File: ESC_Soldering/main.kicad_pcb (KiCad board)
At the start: 2 copper layers, 172 x 77 mm, 29 parts, among them P1 CONN_02X03, P2 CONN_01X03, P3 CONN_01X03, P4 CONN_01X02, P5 CONN_02X05, Q1 BC847CE6327HTSA1, Q2 BC847CE6327HTSA1, U1 PCA9698, U2 ADS7828, U3 AUIPS7111S, U4 AUIPS7111S, U5 74LVC1G08, U6 74LVC1G08, U7 Littlebee, U8 Littlebee

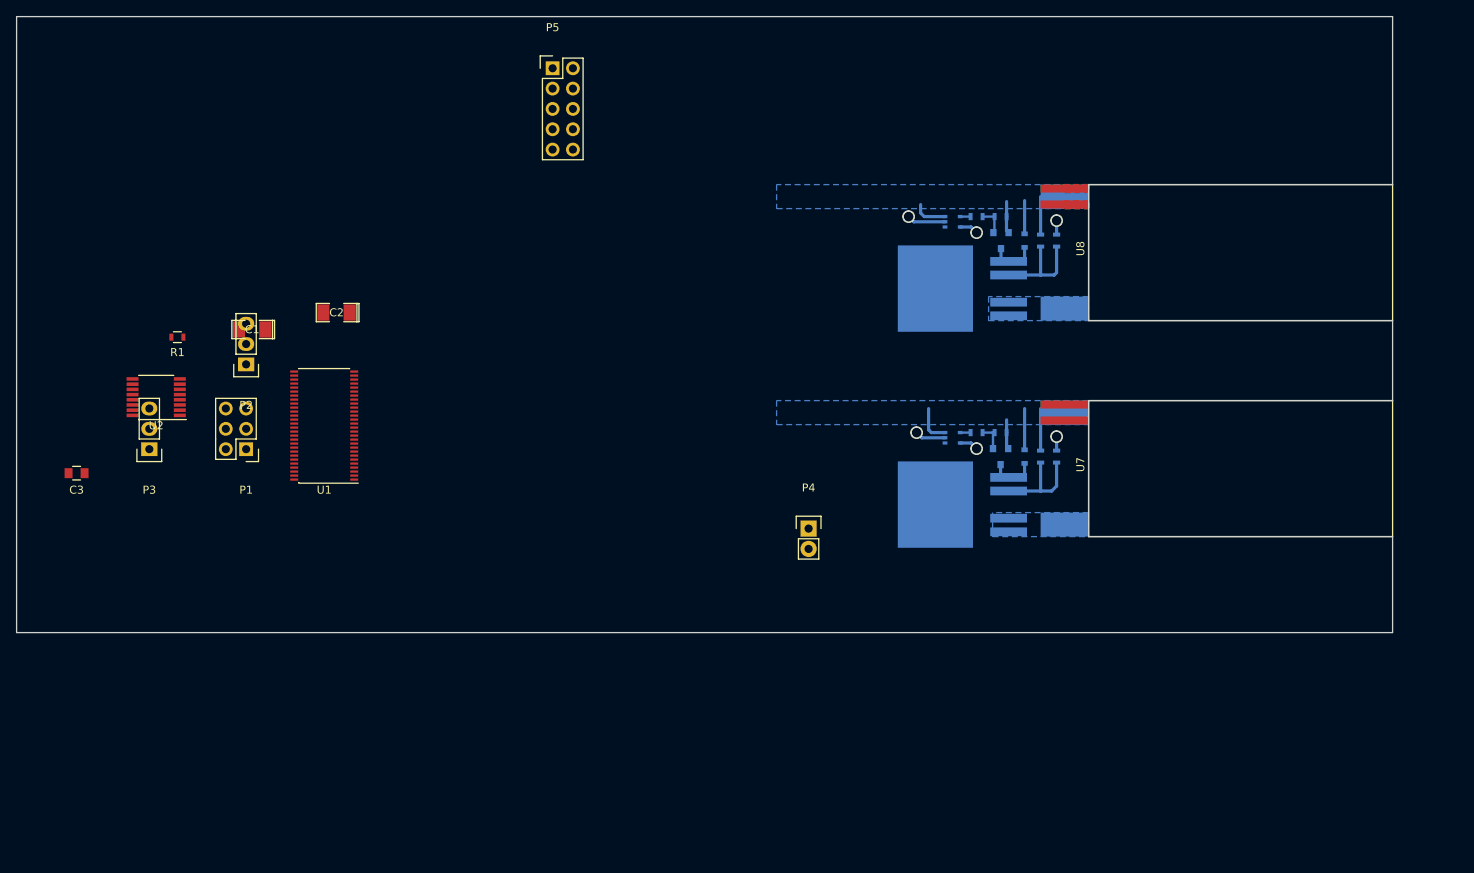
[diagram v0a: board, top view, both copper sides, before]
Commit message: test
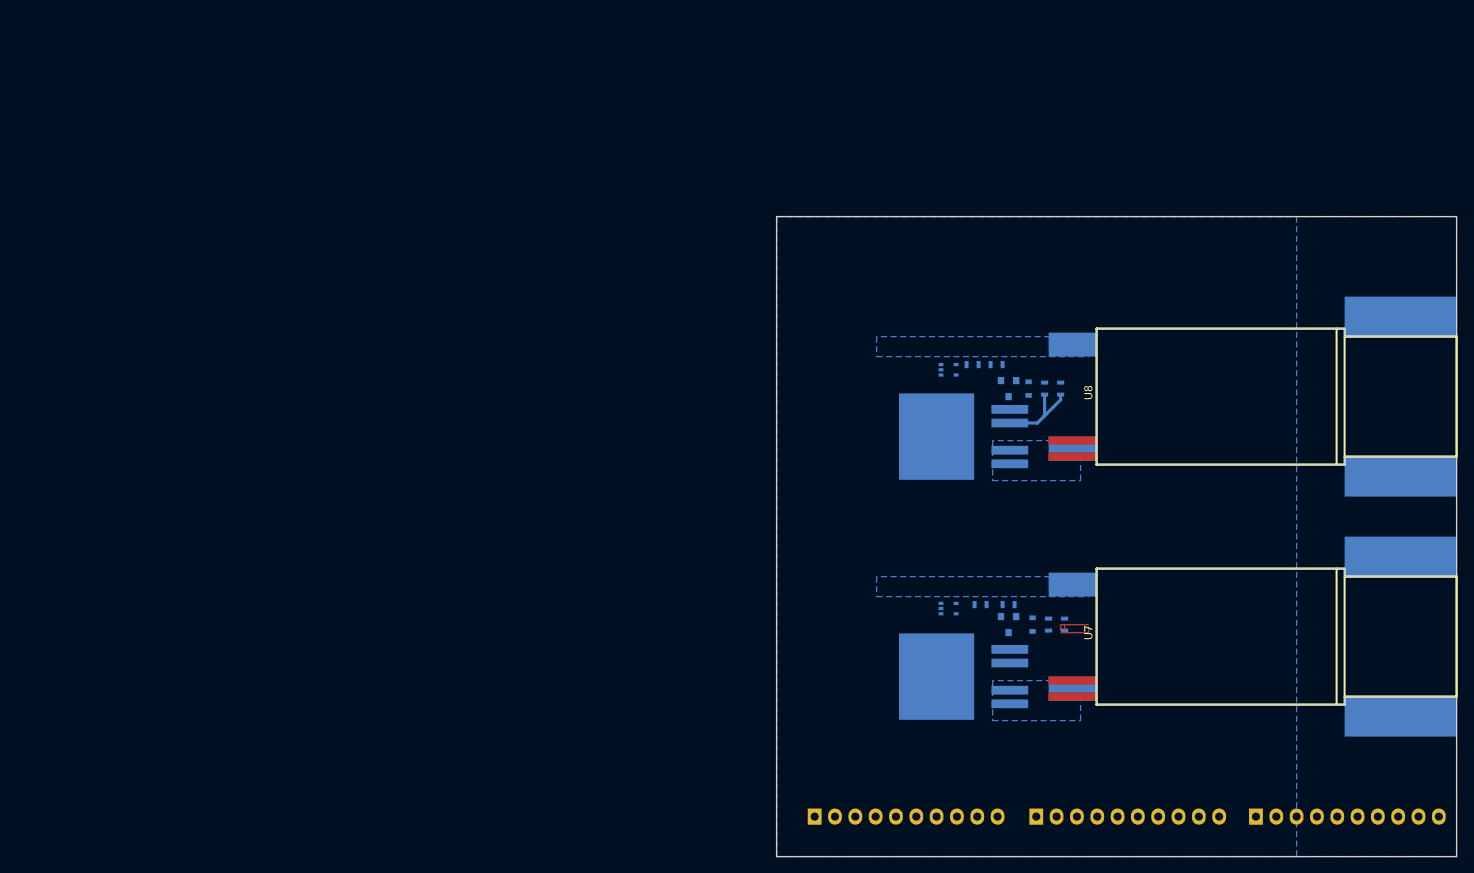
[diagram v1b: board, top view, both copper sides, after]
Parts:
- removed C1, C2: CP, SMD_Packages:SMD-1206_Pol
- removed C3: C, Capacitors_SMD:C_0805
- removed P1: CONN_02X03, Pin_Headers:Pin_Header_Straight_2x03
- removed P2, P3: CONN_01X03, Pin_Headers:Pin_Header_Straight_1x03
- removed P4: CONN_01X02, Pin_Headers:Pin_Header_Straight_1x02
- removed R1: R, Resistors_SMD:R_0603
- removed U1: PCA9698, Housings_SSOP:TSSOP-56_6.1x14mm_Pitch0.5mm
- removed U2: ADS7828, Housings_SSOP:TSSOP-16_4.4x5mm_Pitch0.65mm
- added P6: CONN_01X10, Pin_Headers:Pin_Header_Straight_1x10, B.Cu at (244.9, 160.0)
- added P7: CONN_01X10, Pin_Headers:Pin_Header_Straight_1x10, B.Cu at (189.8, 160.0)
- P5: value CONN_02X05 -> CONN_01X10; footprint Pin_Headers:Pin_Header_Straight_2x05 -> Pin_Headers:Pin_Header_Straight_1x10; moved to B.Cu
- U8: footprint Littlebee -> KiCad-Dev:Littlebee
- moved P5 111.4 mm to (217.5, 160.0), turned to 270 degrees
- moved R3 21.5 mm to (214.0, 133.5)
- moved R2 21.5 mm to (210.5, 133.5)
- moved U3 21.5 mm to (214.2, 142.5)
- moved U5 21.4 mm to (206.5, 134.0)
- moved D1 21.0 mm to (217.0, 136.0)
- moved Q1 21.0 mm to (214.0, 136.0)
- moved R4 21.0 mm to (221.0, 136.0)
- moved R5 21.0 mm to (219.0, 136.0)
- moved U7 21.0 mm to (225.0, 146.0)
- moved Q2 18.5 mm to (214.0, 106.5)
- moved D2 18.5 mm to (216.5, 106.5)
- moved R6 18.5 mm to (209.5, 103.5)
- moved R7 18.5 mm to (212.5, 103.5)
- moved R8 18.5 mm to (220.5, 106.5)
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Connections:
- net /pwr_mod_1/Pwr_Out renamed /pwr_mod_1/Power_Out
- net /pwr_mod_2/Pwr_Out renamed /pwr_mod_2/Power_Out
- P5 pad 1: (no net) -> /Enable_1
- P5 pad 2: (no net) -> /Enable_2
- P5 pad 3: /PWM1 -> (no net)
- R4 pad 2: /pwr_mod_1/Current_Feedback -> /CH1
- R8 pad 2: /pwr_mod_2/Current_Feedback -> /CH2
- U5 pad 1: /pwr_mod_1/Power_Enable_A -> /Enable_1
- U6 pad 1: /pwr_mod_2/Power_Enable_A -> /Enable_2
- U7 pad 4: /pwr_mod_1/Power_Enable_A -> /PWM1
- U8 pad 4: /pwr_mod_2/Power_Enable_A -> /PWM2
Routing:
- net GND: track 36.1 -> 0.01 mm
- net Net-(R4-Pad1): track 12.7 -> 0.00 mm
- net /pwr_mod_1/Power_Enanle_B: track 8.64 -> 0.00 mm, vias 2 -> 0
- net Net-(D1-Pad1): track 6.19 -> 0.00 mm
- net Net-(D2-Pad1): track 6.12 -> 0.00 mm
- net +3V3: track 4.68 -> 0.00 mm, vias 2 -> 0
- net Net-(Q2-Pad1): track 3.56 -> 0.03 mm
- net Net-(Q1-Pad1): track 3.52 -> 0.00 mm
- net Net-(R8-Pad1): track 12.9 -> 11.0 mm
- net /pwr_mod_2/Current_Feedback: track 1.75 -> 0.00 mm, vias 1 -> 0
- net /pwr_mod_1/Current_Feedback: track 1.75 -> 0.00 mm, vias 1 -> 0
- net Net-(R6-Pad2): track 1.30 -> 0.00 mm
- net Net-(R2-Pad2): track 1.30 -> 0.00 mm
- added copper zone on B.Cu, net (none)
- added copper zone on F.Cu, net (none)
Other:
- board size 172 x 77 mm -> 85 x 80 mm
- net class Default: via_dia 1.6 -> 1.3; via_drill 1.2 -> 1
